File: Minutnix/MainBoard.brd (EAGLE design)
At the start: 222.3 x 73.3 mm, 121 parts, among them IC3 TP4056, IC7 FT232RL, Q4 32.768kHz, X1 FH12-12S-0.5S_THINNER, X2 JST-XH-03-PIN-LONG-PAD, X4 JST-XH-03-PIN-LONG-PAD

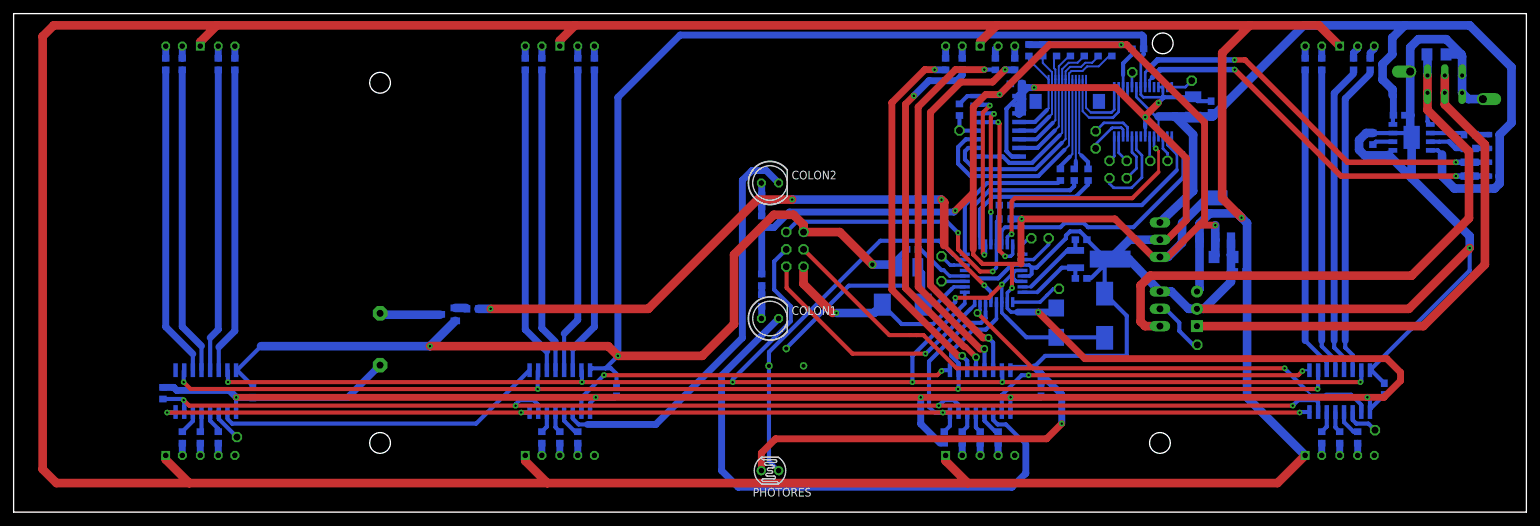
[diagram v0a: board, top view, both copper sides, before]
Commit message: Revert "Revert "Pools of gnd""
This reverts commit 2f73202806bed85f49afe26d98c16d19bdefccd4.
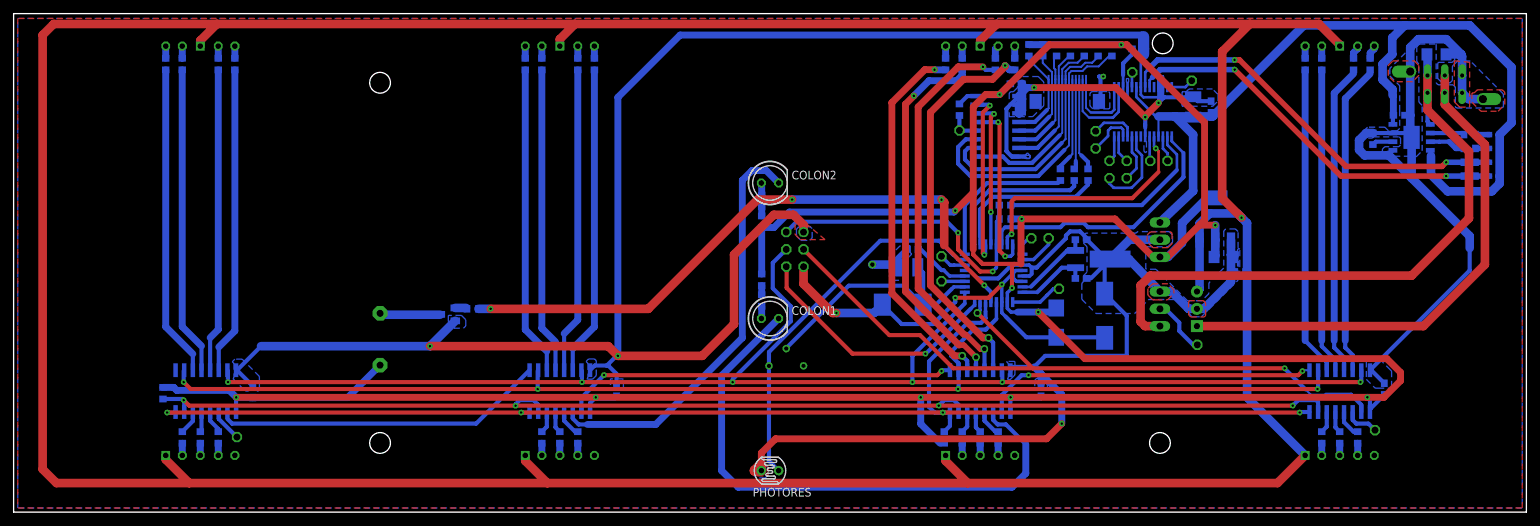
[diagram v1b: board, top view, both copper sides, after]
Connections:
- net GND: now also X1.CASE1, X1.CASE2
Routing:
- net GND: track 664.6 -> 602.3 mm
- net VDD: track 559.9 -> 561.1 mm
- net MS_B: track 57.2 -> 57.8 mm
- net +5V: track 143.6 -> 144.1 mm
- net MS_A: track 56.7 -> 57.2 mm
- net N$43: track 56.0 -> 56.5 mm
- added copper zone on layer 1, net GND
- added copper zone on layer 16, net GND
